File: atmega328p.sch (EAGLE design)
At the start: 8 parts, among them IC1 ATMEGA328-20P, X1 CRYSTALS-NOGND-HC49

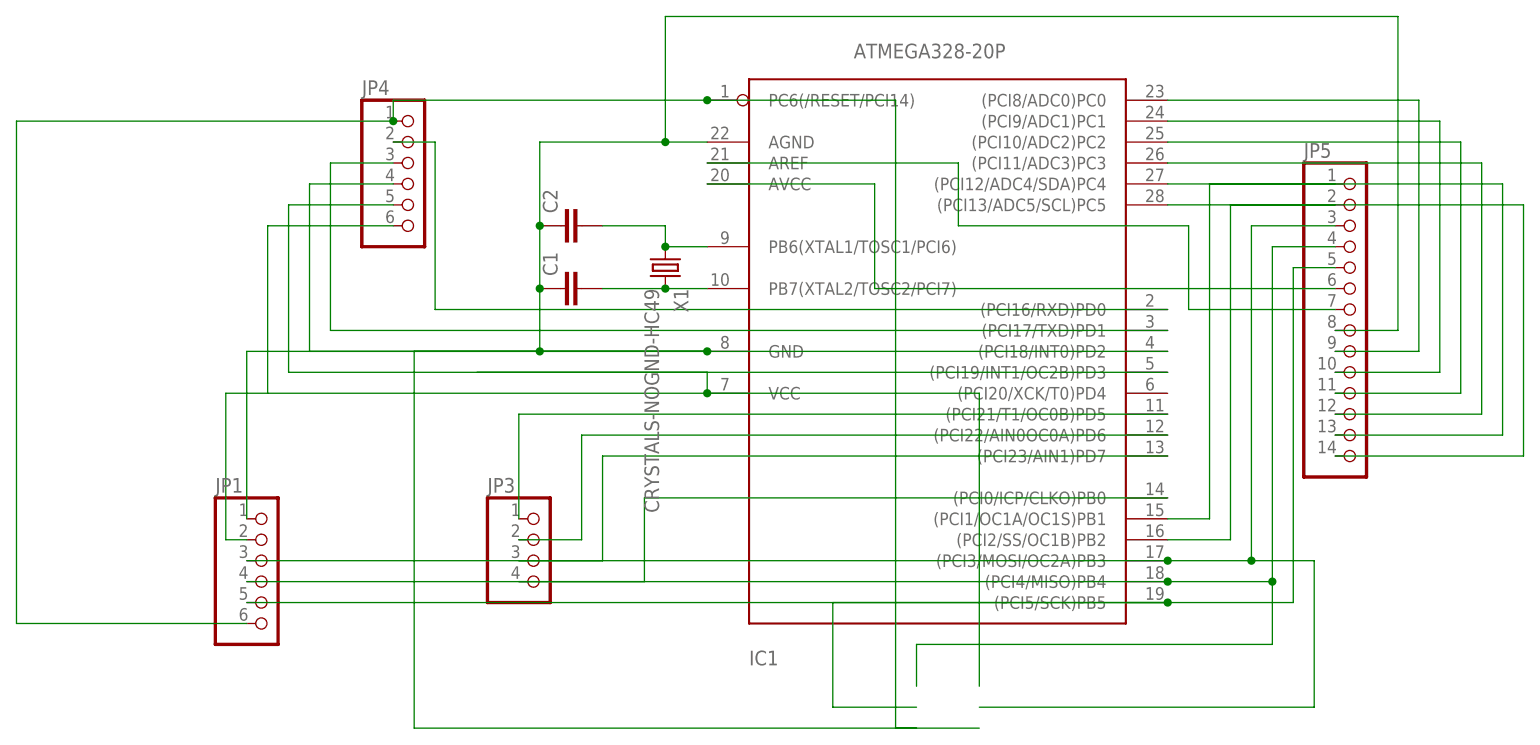
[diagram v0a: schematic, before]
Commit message: with pdf
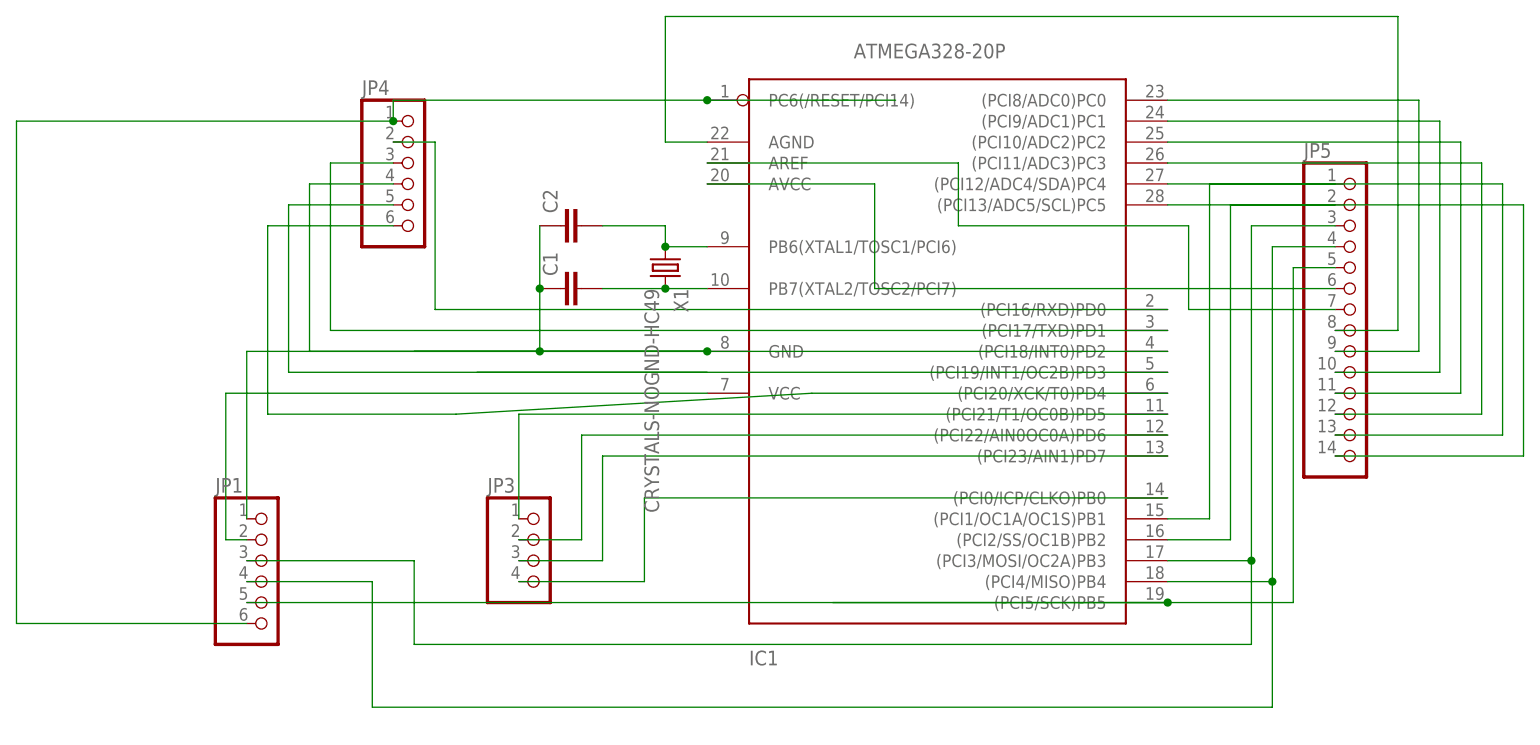
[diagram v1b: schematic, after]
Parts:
- C1: device capacitor-wima:C2.5/2 -> capacitor-wima:C5/2.5
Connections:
- new net N$30: IC1.AGND, JP5.8
- net N$13: now also IC1.(PCI20/XCK/T0)PD4
- net N$5: no longer IC1.AGND, JP5.8
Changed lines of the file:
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@@
 <parts>
 <part name="IC1" library="atmega328" deviceset="ATMEGA328*P" device="" technology="-20"/>
-<part name="C1" library="capacitor-wima" library_urn="urn:adsk.eagle:library:116" deviceset="C" device="2.5/2" package3d_urn="urn:adsk.eagle:package:5415/1"/>
 <part name="C2" library="capacitor-wima" library_urn="urn:adsk.eagle:library:116" deviceset="C" device="2.5/2" package3d_urn="urn:adsk.eagle:package:5415/1"/>
 <part name="X1" library="IQD-Frequency-Products" library_urn="urn:adsk.eagle:library:90" deviceset="CRYSTALS-NOGND" device="-HC49" package3d_urn="urn:adsk.eagle:package:3356/1"/>
@@
 <part name="JP5" library="pinhead" library_urn="urn:adsk.eagle:library:325" deviceset="PINHD-1X14" device="" package3d_urn="urn:adsk.eagle:package:22417/2"/>
 <part name="JP1" library="pinhead" library_urn="urn:adsk.eagle:library:325" deviceset="PINHD-1X6" device="" package3d_urn="urn:adsk.eagle:package:22472/2"/>
+<part name="C1" library="capacitor-wima" library_urn="urn:adsk.eagle:library:116" deviceset="C" device="5/2.5" package3d_urn="urn:adsk.eagle:package:5426/1"/>
 </parts>
 <sheets>
@@
 <instances>
 <instance part="IC1" gate="G$1" x="106.68" y="30.48"/>
-<instance part="C1" gate="G$1" x="66.04" y="35.56" rot="R90"/>
 <instance part="C2" gate="G$1" x="66.04" y="43.18" rot="R90"/>
 <instance part="X1" gate="G$1" x="78.74" y="38.1" rot="R270"/>
@@
 <instance part="JP5" gate="A" x="162.56" y="33.02"/>
 <instance part="JP1" gate="A" x="30.48" y="0"/>
+<instance part="C1" gate="G$1" x="66.04" y="35.56" rot="R90"/>
 </instances>
 <busses>
@@
 <net name="N$4" class="0">
 <segment>
-<pinref part="C1" gate="G$1" pin="2"/>
 <pinref part="X1" gate="G$1" pin="2"/>
 <wire x1="71.12" y1="35.56" x2="78.74" y2="35.56" width="0.1524" layer="91"/>
@@
 <wire x1="78.74" y1="35.56" x2="83.82" y2="35.56" width="0.1524" layer="91"/>
 <junction x="78.74" y="35.56"/>
+<pinref part="C1" gate="G$1" pin="2"/>
 </segment>
 </net>
@@
 <segment>
 <pinref part="C2" gate="G$1" pin="1"/>
-<pinref part="C1" gate="G$1" pin="1"/>
-<wire x1="63.5" y1="43.18" x2="63.5" y2="35.56" width="0.1524" layer="91"/>
 <pinref part="IC1" gate="G$1" pin="GND"/>
 <wire x1="63.5" y1="27.94" x2="83.82" y2="27.94" width="0.1524" layer="91"/>
+<junction x="63.5" y="27.94"/>
+<wire x1="63.5" y1="43.18" x2="63.5" y2="35.56" width="0.1524" layer="91"/>
 <wire x1="63.5" y1="35.56" x2="63.5" y2="27.94" width="0.1524" layer="91"/>
-<junction x="63.5" y="35.56"/>
-<junction x="63.5" y="27.94"/>
-<pinref part="IC1" gate="G$1" pin="AGND"/>
-<wire x1="83.82" y1="53.34" x2="78.74" y2="53.34" width="0.1524" layer="91"/>
-<wire x1="78.74" y1="53.34" x2="63.5" y2="53.34" width="0.1524" layer="91"/>
-<wire x1="63.5" y1="53.34" x2="63.5" y2="43.18" width="0.1524" layer="91"/>
-<junction x="63.5" y="43.18"/>
-<wire x1="116.84" y1="-17.78" x2="48.26" y2="-17.78" width="0.1524" layer="91"/>
-<wire x1="48.26" y1="-17.78" x2="48.26" y2="27.94" width="0.1524" layer="91"/>
 <wire x1="48.26" y1="27.94" x2="63.5" y2="27.94" width="0.1524" layer="91"/>
-<pinref part="JP5" gate="A" pin="8"/>
-<wire x1="160.02" y1="30.48" x2="167.64" y2="30.48" width="0.1524" layer="91"/>
-<wire x1="167.64" y1="30.48" x2="167.64" y2="68.58" width="0.1524" layer="91"/>
-<wire x1="167.64" y1="68.58" x2="78.74" y2="68.58" width="0.1524" layer="91"/>
-<wire x1="78.74" y1="68.58" x2="78.74" y2="53.34" width="0.1524" layer="91"/>
-<junction x="78.74" y="53.34"/>
 <wire x1="83.82" y1="27.94" x2="27.94" y2="27.94" width="0.1524" layer="91"/>
 <junction x="83.82" y="27.94"/>
 <pinref part="JP1" gate="A" pin="1"/>
 <wire x1="27.94" y1="27.94" x2="27.94" y2="7.62" width="0.1524" layer="91"/>
+<pinref part="C1" gate="G$1" pin="1"/>
+<junction x="63.5" y="35.56"/>
 </segment>
 </net>
 <net name="N$7" class="0">
 <segment>
-<wire x1="109.22" y1="-17.78" x2="106.68" y2="-17.78" width="0.1524" layer="91"/>
-<wire x1="106.68" y1="-17.78" x2="106.68" y2="58.42" width="0.1524" layer="91"/>
 <pinref part="IC1" gate="G$1" pin="PC6(/RESET/PCI14)"/>
 <wire x1="106.68" y1="58.42" x2="83.82" y2="58.42" width="0.1524" layer="91"/>
@@
 <pinref part="IC1" gate="G$1" pin="(PCI3/MOSI/OC2A)PB3"/>
 <wire x1="139.7" y1="2.54" x2="149.86" y2="2.54" width="0.1524" layer="91"/>
-<wire x1="149.86" y1="2.54" x2="157.48" y2="2.54" width="0.1524" layer="91"/>
-<wire x1="157.48" y1="2.54" x2="157.48" y2="-15.24" width="0.1524" layer="91"/>
-<wire x1="157.48" y1="-15.24" x2="116.84" y2="-15.24" width="0.1524" layer="91"/>
 <pinref part="JP5" gate="A" pin="3"/>
 <wire x1="160.02" y1="43.18" x2="149.86" y2="43.18" width="0.1524" layer="91"/>
 <wire x1="149.86" y1="43.18" x2="149.86" y2="2.54" width="0.1524" layer="91"/>
+<pinref part="JP1" gate="A" pin="3"/>
+<wire x1="27.94" y1="2.54" x2="48.26" y2="2.54" width="0.1524" layer="91"/>
+<wire x1="48.26" y1="2.54" x2="48.26" y2="-7.62" width="0.1524" layer="91"/>
+<wire x1="48.26" y1="-7.62" x2="149.86" y2="-7.62" width="0.1524" layer="91"/>
+<wire x1="149.86" y1="-7.62" x2="149.86" y2="2.54" width="0.1524" layer="91"/>
 <junction x="149.86" y="2.54"/>
-<pinref part="JP1" gate="A" pin="3"/>
-<wire x1="139.7" y1="2.54" x2="27.94" y2="2.54" width="0.1524" layer="91"/>
-<junction x="139.7" y="2.54"/>
-</segment>
-</net>
-<net name="N$9" class="0">
-<segment>
-<pinref part="IC1" gate="G$1" pin="(PCI4/MISO)PB4"/>
-<wire x1="139.7" y1="0" x2="152.4" y2="0" width="0.1524" layer="91"/>
-<wire x1="152.4" y1="0" x2="152.4" y2="-7.62" width="0.1524" layer="91"/>
-<wire x1="152.4" y1="-7.62" x2="109.22" y2="-7.62" width="0.1524" layer="91"/>
-<wire x1="109.22" y1="-7.62" x2="109.22" y2="-12.7" width="0.1524" layer="91"/>
-<pinref part="JP5" gate="A" pin="4"/>
-<wire x1="160.02" y1="40.64" x2="152.4" y2="40.64" width="0.1524" layer="91"/>
-<wire x1="152.4" y1="40.64" x2="152.4" y2="0" width="0.1524" layer="91"/>
-<junction x="152.4" y="0"/>
-<pinref part="JP1" gate="A" pin="4"/>
-<wire x1="139.7" y1="0" x2="27.94" y2="0" width="0.1524" layer="91"/>
-<junction x="139.7" y="0"/>
 </segment>
 </net>
@@
 <pinref part="IC1" gate="G$1" pin="(PCI5/SCK)PB5"/>
 <wire x1="139.7" y1="-2.54" x2="99.06" y2="-2.54" width="0.1524" layer="91"/>
-<wire x1="99.06" y1="-2.54" x2="99.06" y2="-15.24" width="0.1524" layer="91"/>
-<wire x1="99.06" y1="-15.24" x2="109.22" y2="-15.24" width="0.1524" layer="91"/>
 <pinref part="JP5" gate="A" pin="5"/>
 <wire x1="160.02" y1="38.1" x2="154.94" y2="38.1" width="0.1524" layer="91"/>
@@
 <net name="N$13" class="0">
 <segment>
-<wire x1="30.48" y1="22.86" x2="30.48" y2="43.18" width="0.1524" layer="91"/>
 <pinref part="JP4" gate="A" pin="6"/>
 <wire x1="30.48" y1="43.18" x2="45.72" y2="43.18" width="0.1524" layer="91"/>
+<wire x1="30.48" y1="43.18" x2="30.48" y2="20.32" width="0.1524" layer="91"/>
+<wire x1="30.48" y1="20.32" x2="53.34" y2="20.32" width="0.1524" layer="91"/>
+<wire x1="53.34" y1="20.32" x2="96.52" y2="22.86" width="0.1524" layer="91"/>
+<pinref part="IC1" gate="G$1" pin="(PCI20/XCK/T0)PD4"/>
+<wire x1="96.52" y1="22.86" x2="139.7" y2="22.86" width="0.1524" layer="91"/>
 </segment>
 </net>
@@
 <net name="N$17" class="0">
 <segment>
-<pinref part="JP3" gate="A" pin="4"/>
-<wire x1="60.96" y1="0" x2="76.2" y2="0" width="0.1524" layer="91"/>
 <wire x1="76.2" y1="0" x2="76.2" y2="10.16" width="0.1524" layer="91"/>
 <pinref part="IC1" gate="G$1" pin="(PCI0/ICP/CLKO)PB0"/>
 <wire x1="76.2" y1="10.16" x2="139.7" y2="10.16" width="0.1524" layer="91"/>
+<pinref part="JP3" gate="A" pin="4"/>
+<wire x1="76.2" y1="0" x2="60.96" y2="0" width="0.1524" layer="91"/>
 </segment>
 </net>
@@
 <wire x1="27.94" y1="5.08" x2="25.4" y2="5.08" width="0.1524" layer="91"/>
 <pinref part="IC1" gate="G$1" pin="VCC"/>
-<wire x1="55.88" y1="25.4" x2="83.82" y2="25.4" width="0.1524" layer="91"/>
-<wire x1="83.82" y1="25.4" x2="83.82" y2="22.86" width="0.1524" layer="91"/>
-<wire x1="116.84" y1="22.86" x2="83.82" y2="22.86" width="0.1524" layer="91"/>
-<junction x="83.82" y="22.86"/>
-<wire x1="116.84" y1="-12.7" x2="116.84" y2="22.86" width="0.1524" layer="91"/>
 <wire x1="25.4" y1="22.86" x2="83.82" y2="22.86" width="0.1524" layer="91"/>
 </segment>
@@
 </segment>
 </net>
+<net name="N$29" class="0">
+<segment>
+<wire x1="55.88" y1="25.4" x2="83.82" y2="25.4" width="0.1524" layer="91"/>
+</segment>
+</net>
+<net name="N$30" class="0">
+<segment>
+<pinref part="IC1" gate="G$1" pin="AGND"/>
+<wire x1="83.82" y1="53.34" x2="78.74" y2="53.34" width="0.1524" layer="91"/>
+<pinref part="JP5" gate="A" pin="8"/>
+<wire x1="160.02" y1="30.48" x2="167.64" y2="30.48" width="0.1524" layer="91"/>
+<wire x1="167.64" y1="30.48" x2="167.64" y2="68.58" width="0.1524" layer="91"/>
+<wire x1="167.64" y1="68.58" x2="78.74" y2="68.58" width="0.1524" layer="91"/>
+<wire x1="78.74" y1="68.58" x2="78.74" y2="53.34" width="0.1524" layer="91"/>
+</segment>
+</net>
+<net name="N$31" class="0">
+<segment>
+<pinref part="JP5" gate="A" pin="4"/>
+<wire x1="160.02" y1="40.64" x2="152.4" y2="40.64" width="0.1524" layer="91"/>
+<wire x1="152.4" y1="40.64" x2="152.4" y2="0" width="0.1524" layer="91"/>
+<pinref part="IC1" gate="G$1" pin="(PCI4/MISO)PB4"/>
+<wire x1="139.7" y1="0" x2="152.4" y2="0" width="0.1524" layer="91"/>
+<pinref part="JP1" gate="A" pin="4"/>
+<wire x1="27.94" y1="0" x2="43.18" y2="0" width="0.1524" layer="91"/>
+<wire x1="43.18" y1="0" x2="43.18" y2="-15.24" width="0.1524" layer="91"/>
+<wire x1="43.18" y1="-15.24" x2="152.4" y2="-15.24" width="0.1524" layer="91"/>
+<wire x1="152.4" y1="-15.24" x2="152.4" y2="0" width="0.1524" layer="91"/>
+<junction x="152.4" y="0"/>
+</segment>
+</net>
